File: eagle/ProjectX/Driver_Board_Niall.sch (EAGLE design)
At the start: 17 parts, among them IC1 LM317MBSTT3, U1 ADA4091-2ARZ-RL, U2 ADA4091-2ARZ-RL

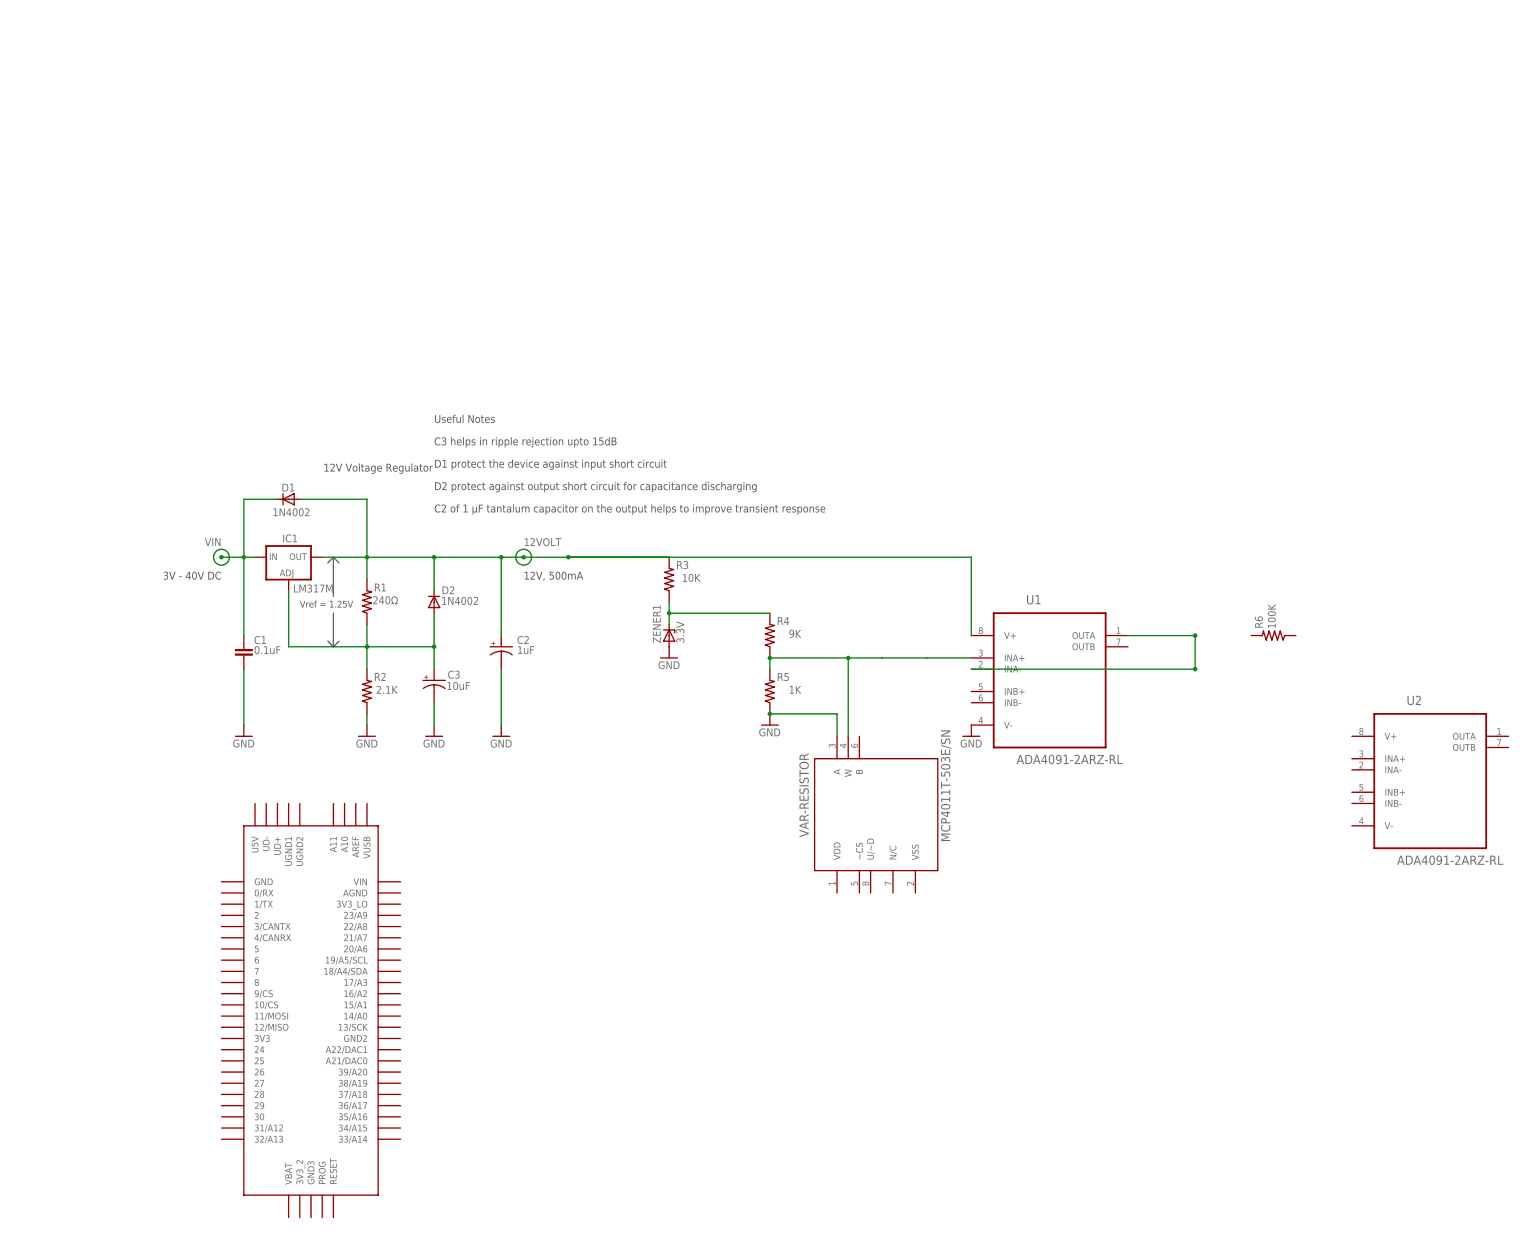
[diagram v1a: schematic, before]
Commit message: Eagle work- niall
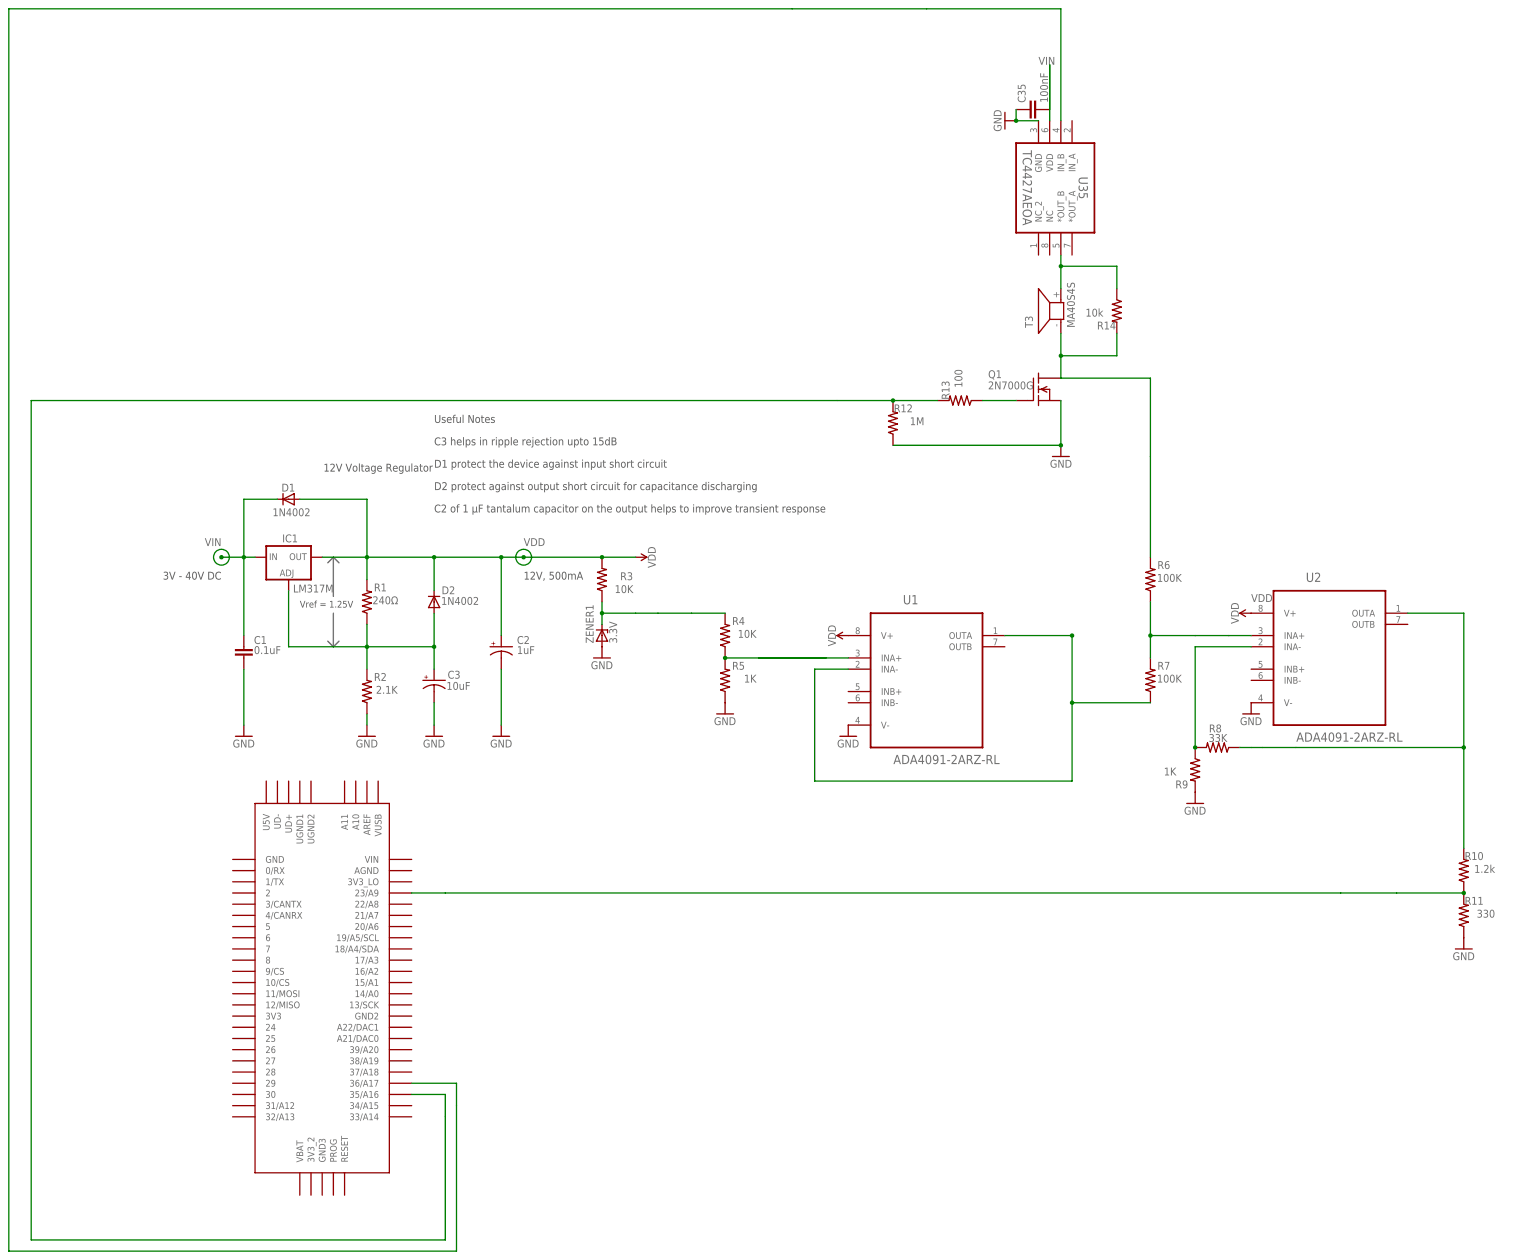
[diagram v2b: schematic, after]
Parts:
- removed VAR-RESISTOR: MCP4011T-503E/SN, SnapEDA-Library:MCP4011T-503E/SN
- added C35: 100nF, resistor:C-EUC0805
- added Q1: 2N7000G, SnapEDA-Library:2N7000G
- added R10: 1.2k, resistor:R-US_M0805
- added R11: 330, resistor:R-US_M0805
- added R12: 1M, resistor:R-US_M0805
- added R13: 100, resistor:R-US_M0805
- added R14: 10k, resistor:R-US_M0805
- added R7: 100K, resistor:R-US_M0805
- added R8: 33K, resistor:R-US_M0805
- added R9: 1K, resistor:R-US_M0805
- added T3: MA40S4S, Parts:MA40S4S
- added U35: TC4427AEOA, Parts:TC4427AEOA
- R4: value 9K -> 10K
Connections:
- removed net 12VOLT: C2.+, D1.A, D2.C, IC1.OUT, R1.2, R3.2, U1.V+
- new net N$10: R12.2, R13.2, U$2.35/A16
- new net N$11: Q1.GATE, R13.1
- new net N$12: R14.2, T3.1
- new net N$13: U$2.36/A17, U35.IN_B
- new net N$5: R6.1, R7.2, U2.INA+
- new net N$6: Q1.DRN, R6.2
- new net N$7: R10.2, R8.1, U2.OUTA
- new net N$72: R14.1, T3.2, U35.*OUT_B
- new net N$8: R8.2, R9.1, U2.INA-
- new net N$9: R10.1, R11.2, U$2.23/A9
- new net VDD: C2.+, D1.A, D2.C, IC1.OUT, R1.2, R3.2, U1.V+, U2.V+
- net GND: now also C35.1, Q1.SRC, R11.1, R12.1, R9.2, U2.V-, U35.GND; no longer VAR-RESISTOR.A
- net N$2: no longer VAR-RESISTOR.W
- net N$4: now also R7.1
- net VIN: now also C35.2, U35.VDD
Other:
- moved on the sheet: R3, R4, R5, R6, U1, U2, ZENER1
